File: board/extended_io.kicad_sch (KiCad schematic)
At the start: 54 parts

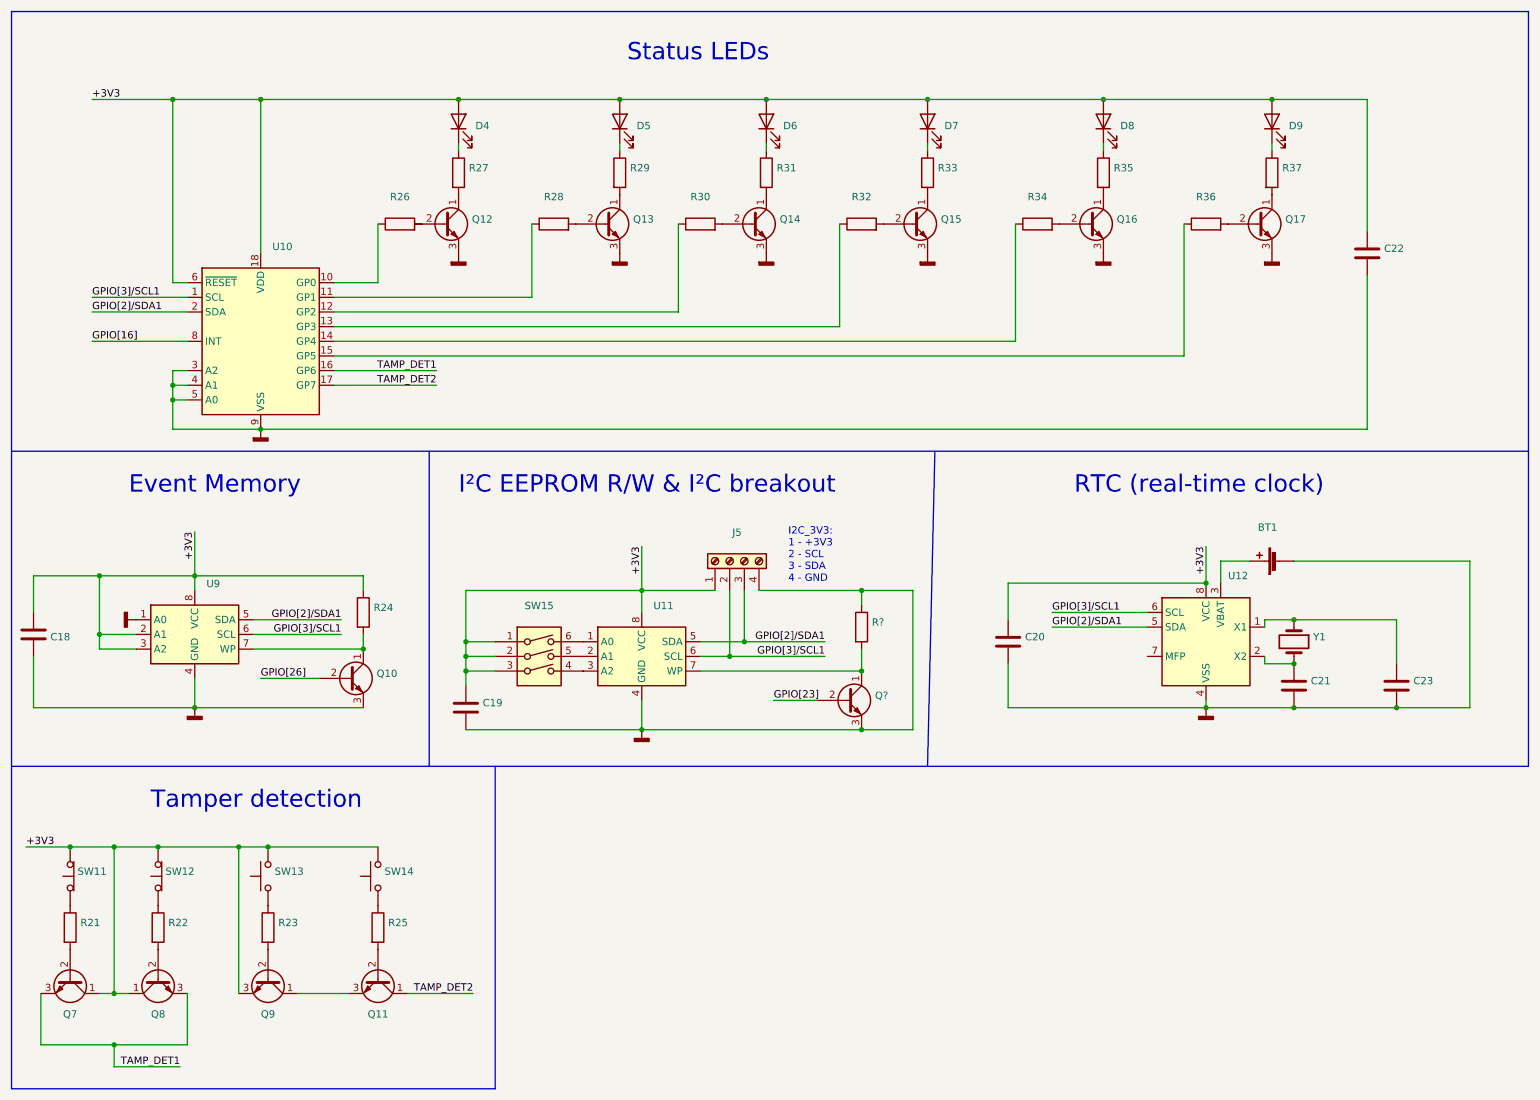
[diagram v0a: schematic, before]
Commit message: Fix voltage regulation circuit.
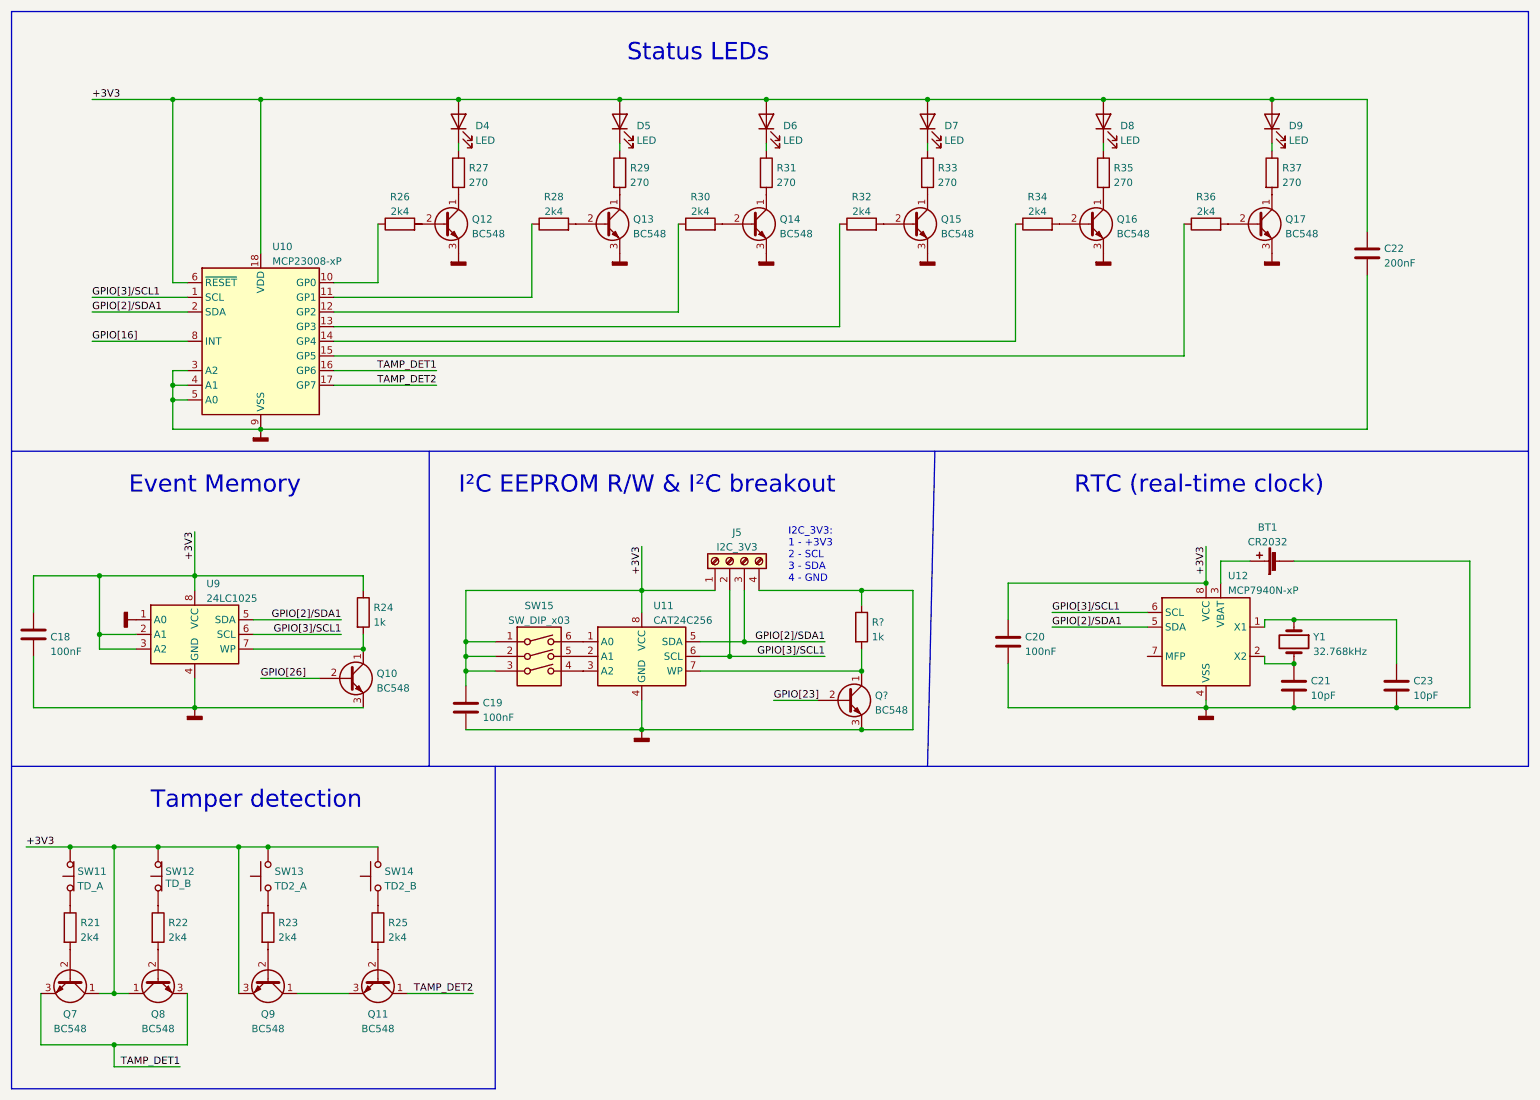
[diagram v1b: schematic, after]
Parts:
- BT1: value (none) -> CR2032
- C18, C19, C20: value (none) -> 100nF
- C21, C23: value (none) -> 10pF
- C22: value (none) -> 200nF
- D4, D5, D6, D7, D8, D9: value (none) -> LED
- J5: value (none) -> I2C_3V3
- Q10, Q11, Q12, Q13, Q14, Q15, Q16, Q17, Q7, Q8, Q9, Q?: value (none) -> BC548; footprint (none) -> Package_TO_SOT_THT:TO-92_Inline
- R21, R22, R23, R25, R26, R28, R30, R32, R34, R36: value (none) -> 2k4
- R24, R?: value (none) -> 1k
- R27, R29, R31, R33, R35, R37: value (none) -> 270
- SW11: value (none) -> TD_A
- SW12: value (none) -> TD_B
- SW13: value (none) -> TD2_A
- SW14: value (none) -> TD2_B
- SW15: value (none) -> SW_DIP_x03
- U10: value (none) -> MCP23008-xP; footprint (none) -> Package_DIP:DIP-18_W7.62mm
- U11: value (none) -> CAT24C256
- U12: value (none) -> MCP7940N-xP; footprint (none) -> Package_DIP:DIP-8_W7.62mm_Socket_LongPads
- U9: value (none) -> 24LC1025
- Y1: value (none) -> 32.768kHz

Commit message: Fix filenames.
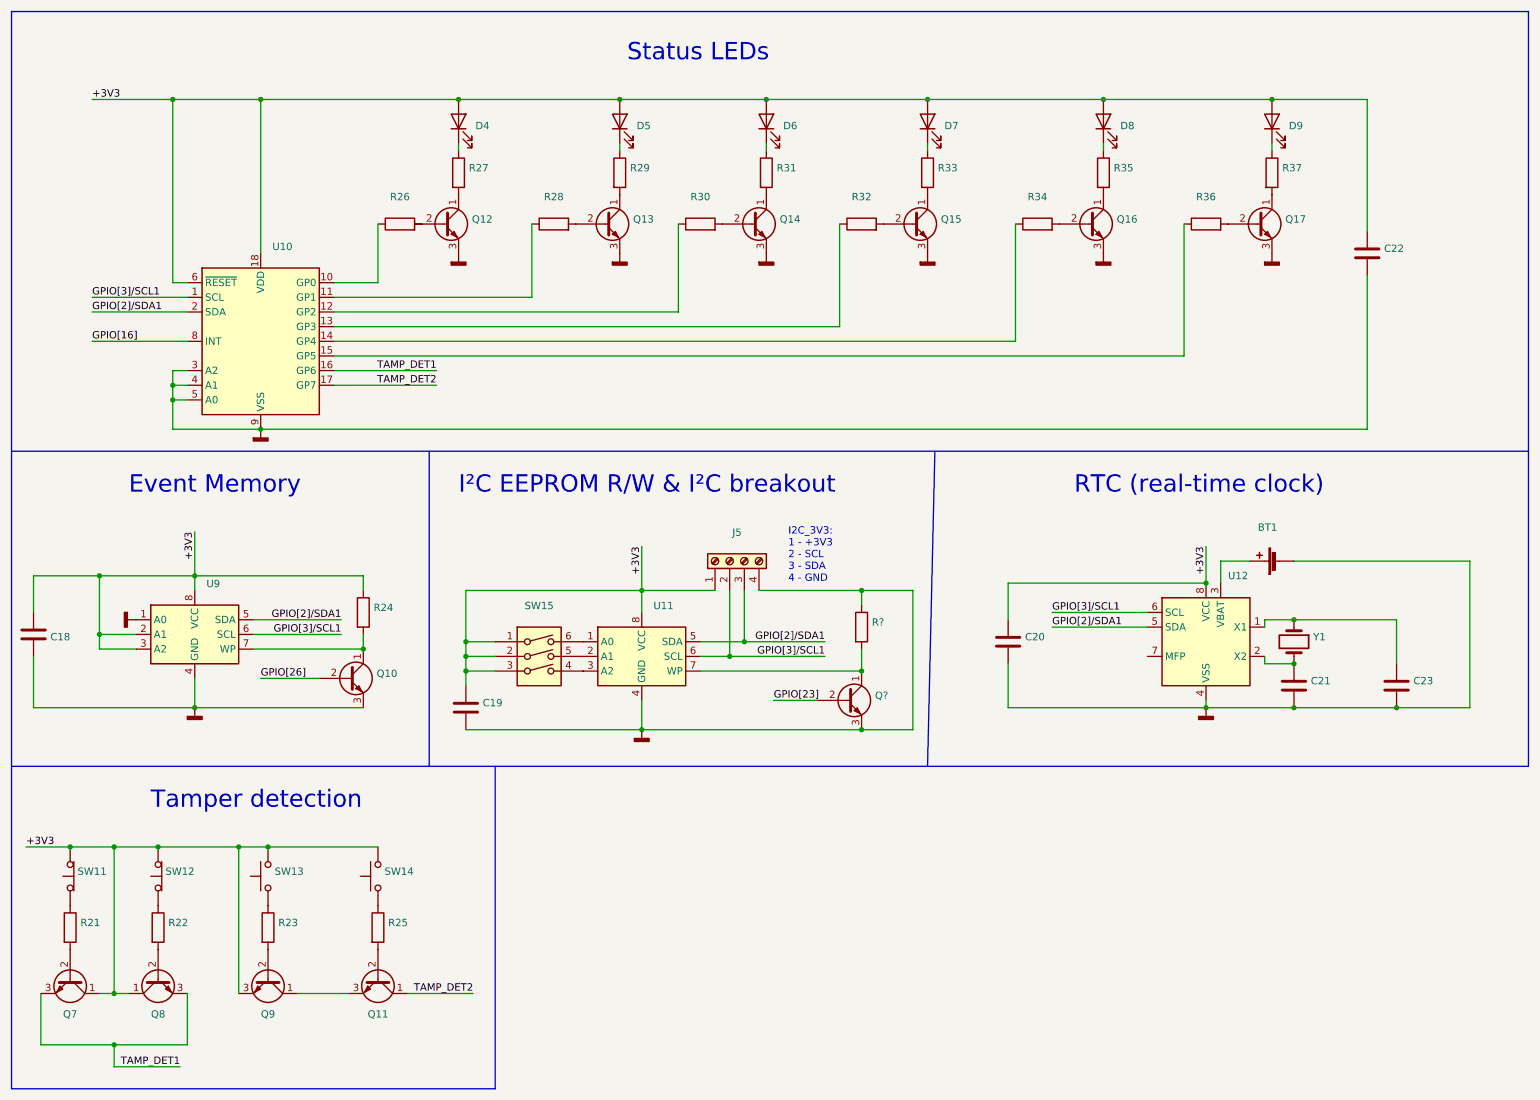
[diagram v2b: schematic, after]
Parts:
- BT1: value CR2032 -> (none)
- C18, C19, C20: value 100nF -> (none)
- C21, C23: value 10pF -> (none)
- C22: value 200nF -> (none)
- D4, D5, D6, D7, D8, D9: value LED -> (none)
- J5: value I2C_3V3 -> (none)
- Q10, Q11, Q12, Q13, Q14, Q15, Q16, Q17, Q7, Q8, Q9, Q?: value BC548 -> (none); footprint Package_TO_SOT_THT:TO-92_Inline -> (none)
- R21, R22, R23, R25, R26, R28, R30, R32, R34, R36: value 2k4 -> (none)
- R24, R?: value 1k -> (none)
- R27, R29, R31, R33, R35, R37: value 270 -> (none)
- SW11: value TD_A -> (none)
- SW12: value TD_B -> (none)
- SW13: value TD2_A -> (none)
- SW14: value TD2_B -> (none)
- SW15: value SW_DIP_x03 -> (none)
- U10: value MCP23008-xP -> (none); footprint Package_DIP:DIP-18_W7.62mm -> (none)
- U11: value CAT24C256 -> (none)
- U12: value MCP7940N-xP -> (none); footprint Package_DIP:DIP-8_W7.62mm_Socket_LongPads -> (none)
- U9: value 24LC1025 -> (none)
- Y1: value 32.768kHz -> (none)
